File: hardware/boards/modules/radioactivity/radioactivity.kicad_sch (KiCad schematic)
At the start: 51 parts, among them J1 jmp1, J2 Programming Header, J3 jmp1, Q1 S8050, Q2 MMBTA42, Q3 S8050, Q4 S8050, T1 74LVC1G17GW, U1 TLC555, U2 TLC555, U3 ATTINY1614

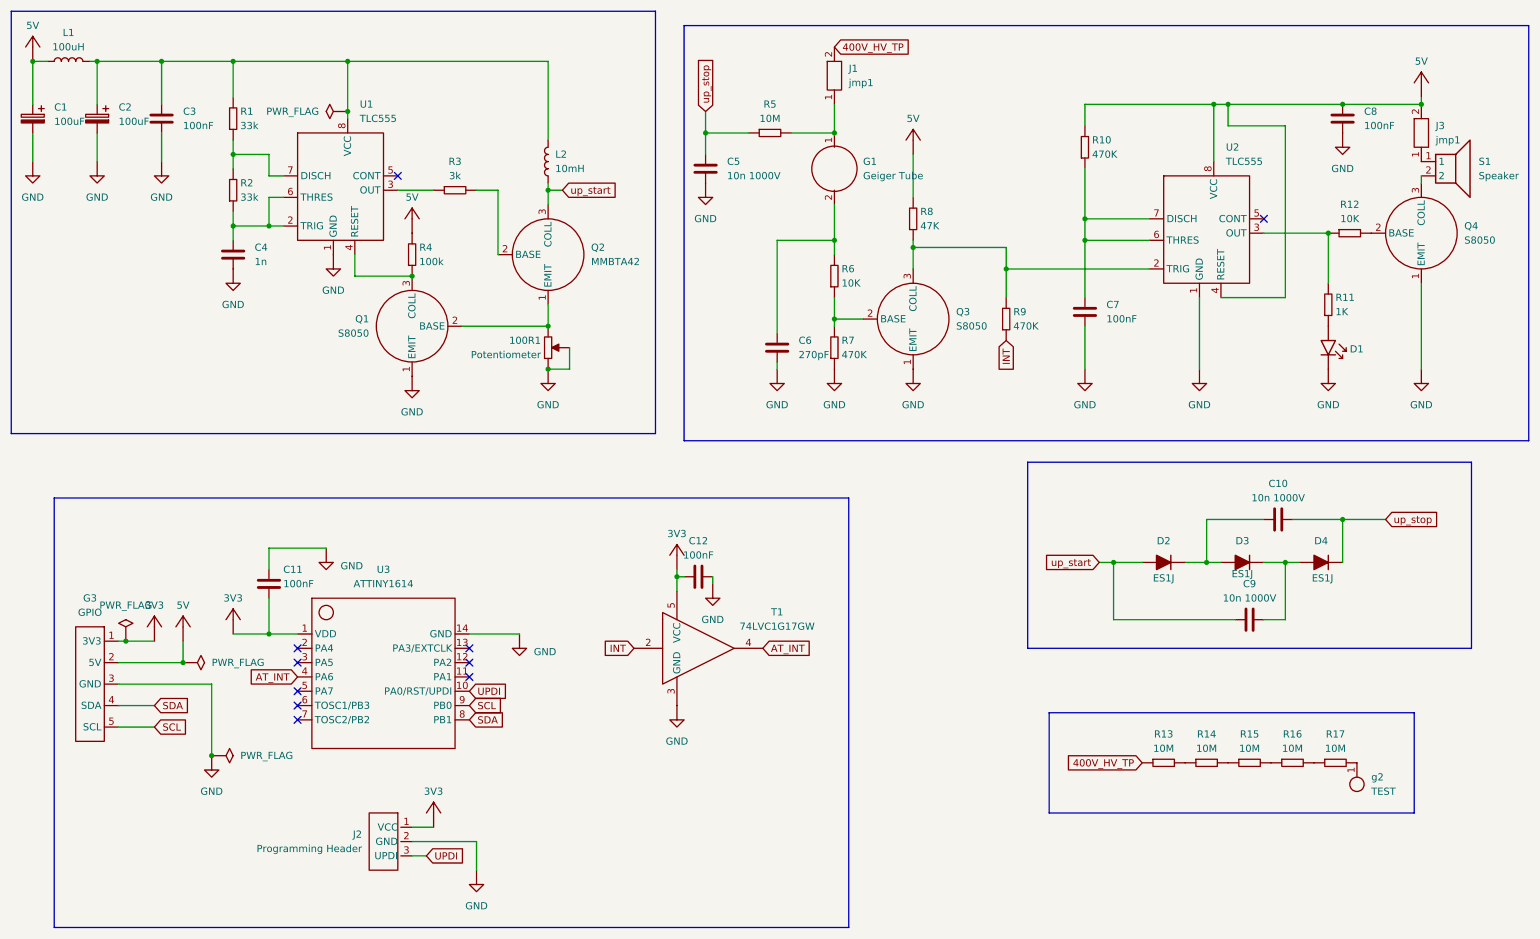
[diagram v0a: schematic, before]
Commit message: finished geiger module pcb
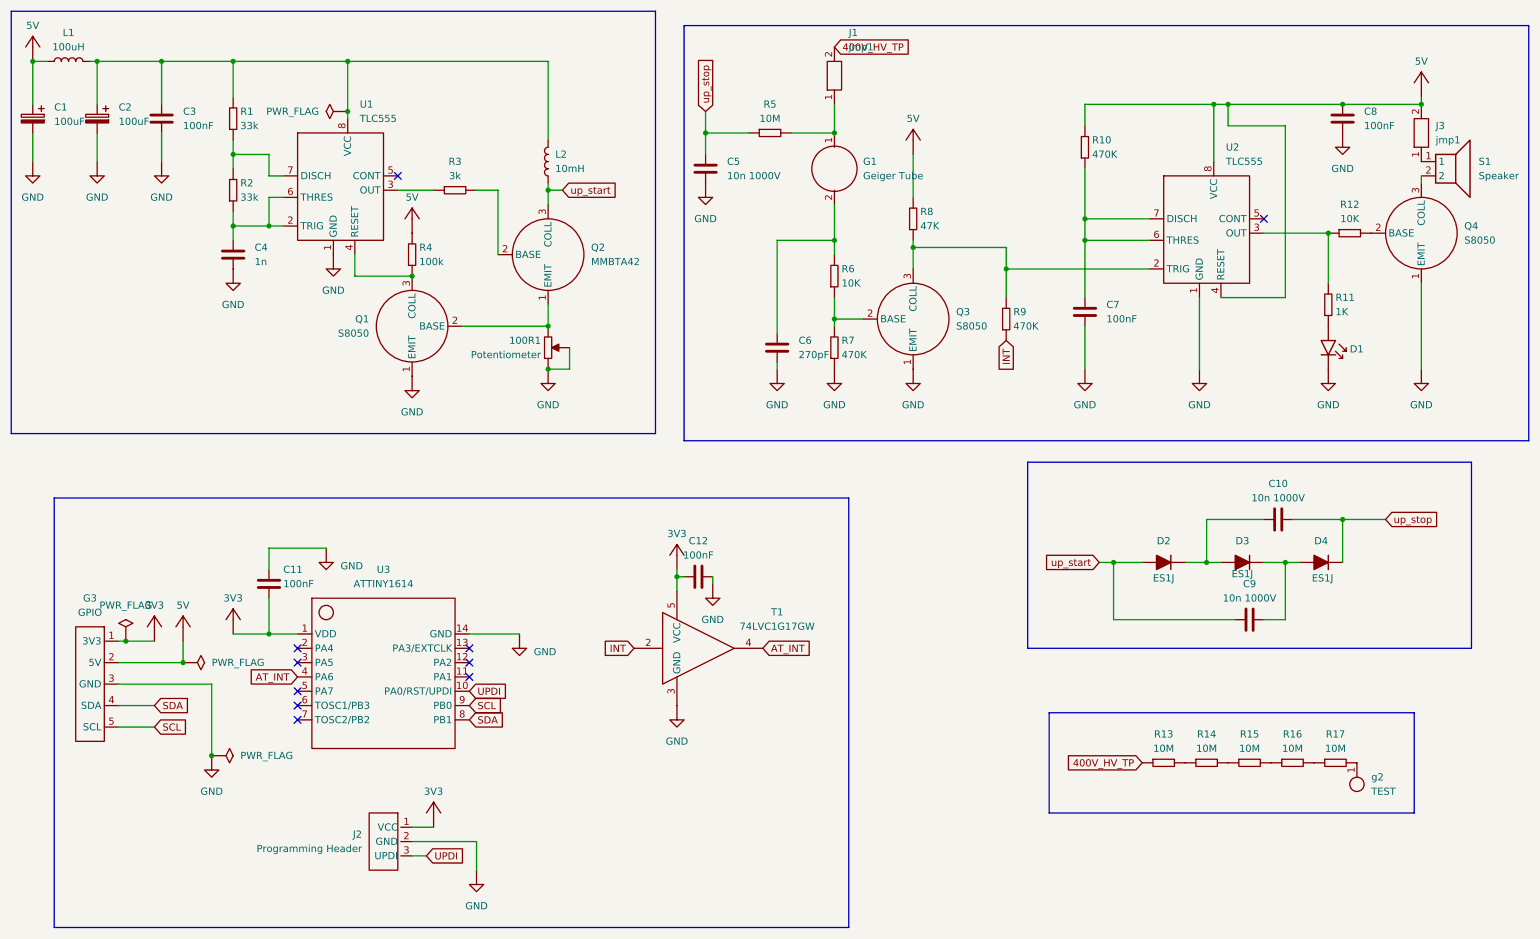
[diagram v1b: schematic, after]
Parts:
- 100R1: footprint (none) -> common:SMD_3P_3.8X3.6
- C1, C2: footprint (none) -> common:C_Elec_SMD_5x5.4
- C10, C5, C9: footprint (none) -> common:C_1206
- C11, C12, C3, C4, C6, C7, C8, L2: footprint (none) -> common:C_0603
- D1: footprint (none) -> common:LED_0603
- D2, D3, D4: footprint (none) -> common:SMA(DO-214AC)
- G1: footprint (none) -> geiger:Geiger_Tube_J305
- G3: footprint (none) -> air_sens_foots:GPIO_HEADER
- J1: footprint (none) -> common:Jumper_2
- J2: footprint (none) -> air_sens_foots:ATtiny_Programming_Header
- J3: footprint (none) -> common:Jumper_2; now in the parts list
- L1: footprint (none) -> common:SMD(7.1x6.6)
- Q1, Q2, Q3, Q4: footprint (none) -> common:SOT-23
- R1, R10, R11, R12, R13, R14, R15, R16, R17, R2, R3, R4, R5, R6, R7, R8, R9: footprint (none) -> common:R_0603
- S1: footprint (none) -> common:buzzer_8.5x8.5
- T1: footprint (none) -> common:SOT353
- U1, U2: footprint (none) -> common:SOIC-8
- U3: footprint (none) -> air_sens_foots:ATtiny1614
- g2: footprint (none) -> air_sens_foots:gpio_1; now in the parts list
